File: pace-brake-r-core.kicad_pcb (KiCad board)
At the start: 2 copper layers, 50 x 50 mm, 22 parts, among them J2 Conn_01x02_Socket, J3 Conn_01x02_Socket, Q1 AOD4184, U1 EG2131, U2 TL432AIDBZR, U3 XL7015E1

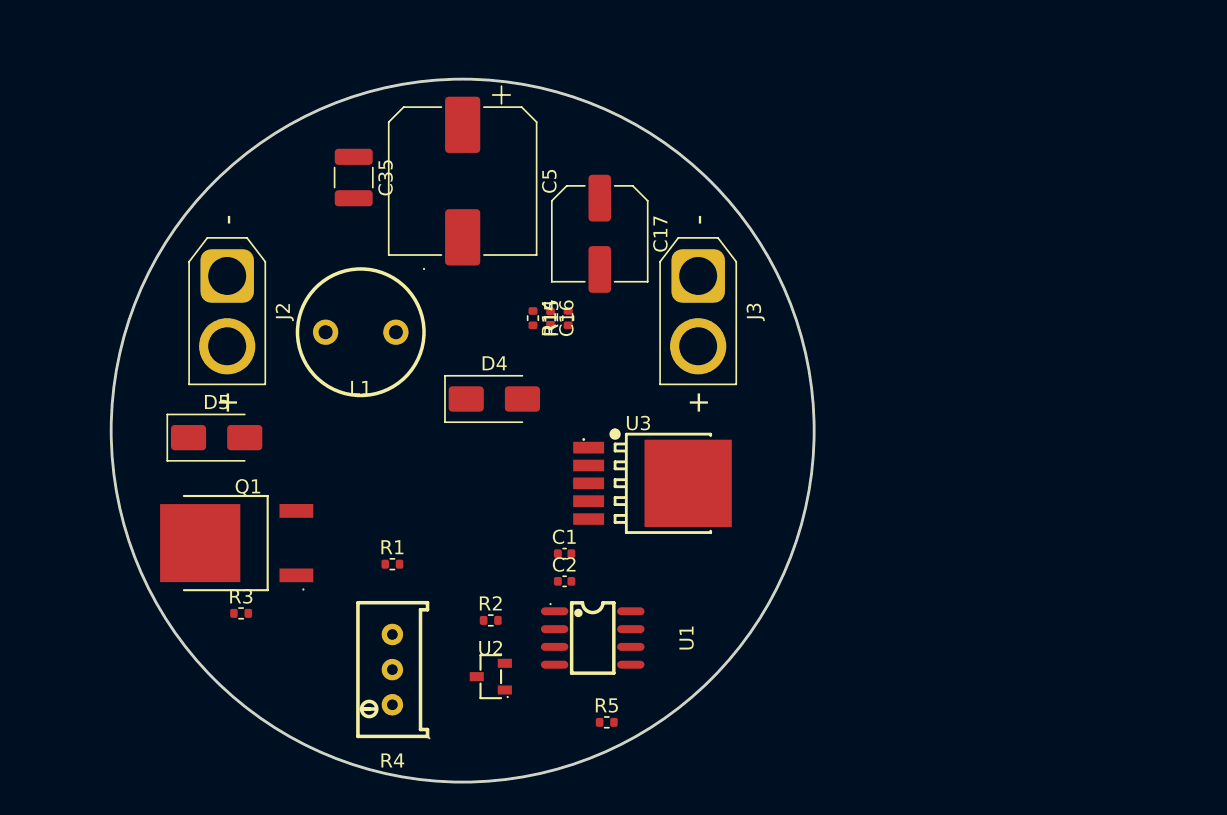
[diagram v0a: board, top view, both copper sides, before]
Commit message: Continue PCB layout progress
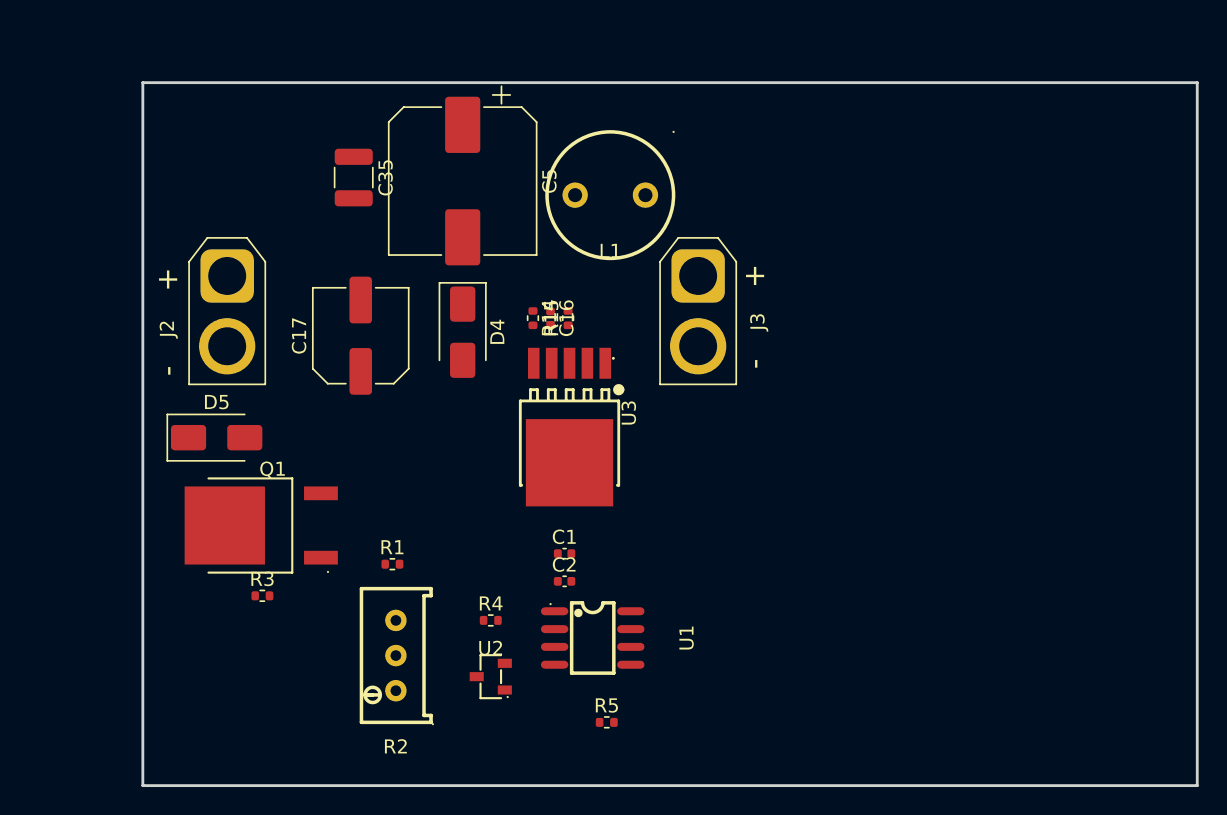
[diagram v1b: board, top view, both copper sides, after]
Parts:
- moved L1 20.3 mm to (158.2, 83.0)
- moved C17 18.5 mm to (140.5, 93.0), turned to 90 degrees
- moved U3 7.00 mm to (155.3, 98.5), turned to -90 degrees
- moved D4 5.26 mm to (147.8, 92.8), turned to -90 degrees
- moved Q1 2.15 mm to (134.2, 106.5)
- moved R3 1.96 mm to (133.5, 111.5)
- moved R2 1.03 mm to (143.0, 115.8)
- renumbered R4 to R2, R2 to R4
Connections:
- net /GATE2 renamed Net-(U1-LO)
- R1 pad 2: Net-(U2-REF) -> Net-(FB1-Pad2)
- R2 pad 2: Net-(U2-REF) -> Net-(FB1-Pad2)
- R5 pad 1: Net-(FB1-Pad1) -> Net-(FB1-Pad2)
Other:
- board size 50 x 50 mm -> 75 x 50 mm
- copper layers 2 -> 4

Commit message: schematic revision changes
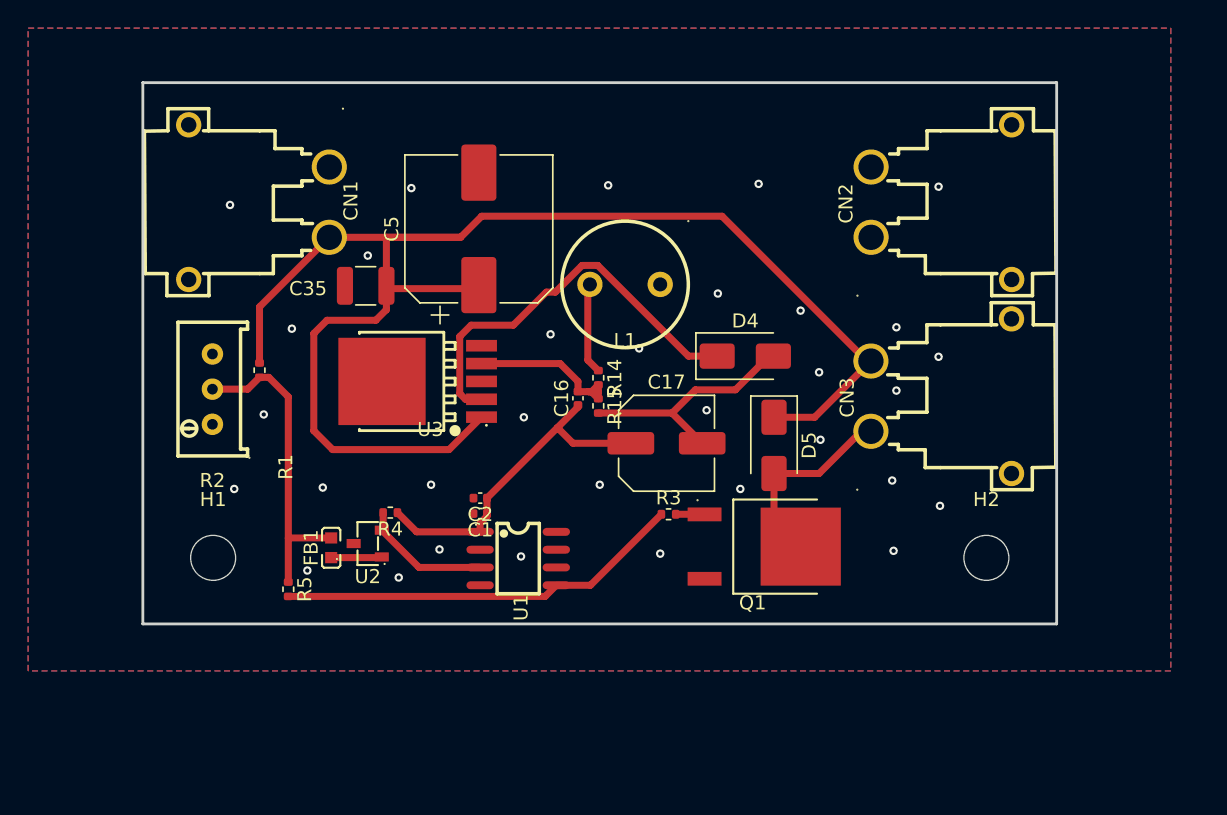
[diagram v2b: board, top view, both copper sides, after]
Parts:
- removed J2, J3: Conn_01x02_Socket, Connector_AMASS:AMASS_XT30U-F_1x02_P5.0mm_Vertical
- added CN1: XT30PW-M, imported-project-library:CONN-TH_XT30PW-M, F.Cu at (133.3, 83.5)
- added CN2: XT30PW-M, imported-project-library:CONN-TH_XT30PW-M, F.Cu at (181.8, 83.5)
- added CN3: XT30PW-M, imported-project-library:CONN-TH_XT30PW-M, F.Cu at (181.8, 97.3)
- added FB1: FerriteBead_Small, imported-project-library:L0603, F.Cu at (138.4, 108.1)
- added H1: MountingHole, MountingHole:MountingHole_3.2mm_M3, F.Cu at (130.0, 108.8)
- added H2: MountingHole, MountingHole:MountingHole_3.2mm_M3, F.Cu at (185.0, 108.8)
- moved D5 39.6 mm to (169.9, 100.8), turned to -90 degrees
- moved Q1 34.2 mm to (168.4, 108.0), turned to 180 degrees
- moved R3 29.5 mm to (162.4, 105.7)
- moved R5 24.6 mm to (135.3, 111.0), turned to -90 degrees
- moved C17 23.1 mm to (162.2, 100.7), turned to 0 degrees
- moved R2 23.0 mm to (129.9, 96.8)
- moved D4 20.2 mm to (167.8, 94.5), turned to 0 degrees
- moved R1 16.7 mm to (133.3, 95.5), turned to -90 degrees
- moved U2 12.9 mm to (141.0, 107.8)
- moved R4 10.5 mm to (142.6, 105.6), turned to 180 degrees
- moved U3 10.1 mm to (145.6, 96.2), turned to 180 degrees
- moved C2 8.43 mm to (149.0, 104.5), turned to 180 degrees
- moved U1 7.75 mm to (151.7, 108.8)
- moved C35 7.75 mm to (140.8, 89.5), turned to 180 degrees
- moved C1 6.64 mm to (149.0, 105.7), turned to 180 degrees
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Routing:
- net VDD: track 0.00 -> 106.8 mm
- net +12V: track 0.00 -> 30.5 mm
- net Net-(U1-LO): track 0.00 -> 29.0 mm
- net Net-(D4-K): track 0.00 -> 28.8 mm
- net Net-(FB1-Pad2): track 0.00 -> 22.6 mm
- net GND: track 0.00 -> 17.2 mm, vias 0 -> 32
- net Net-(CN3--): track 0.00 -> 14.1 mm
- net Net-(U3-FB): track 0.00 -> 12.4 mm
- net Net-(U1-LIN): track 0.00 -> 9.38 mm
- net Net-(U2-REF): track 0.00 -> 3.62 mm
- net Net-(Q1-G): track 0.00 -> 2.05 mm
- added copper zone on B.Cu, net GND
- added copper zone on F.Cu, net GND
- added copper zone on In1.Cu, net GND
- added copper zone on In2.Cu, net GND
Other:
- board size 75 x 50 mm -> 65 x 38.5 mm
